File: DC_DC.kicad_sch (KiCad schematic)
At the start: 22 parts, among them Q1 Q_NMOS_GDS, U1 UC3845_SOIC8

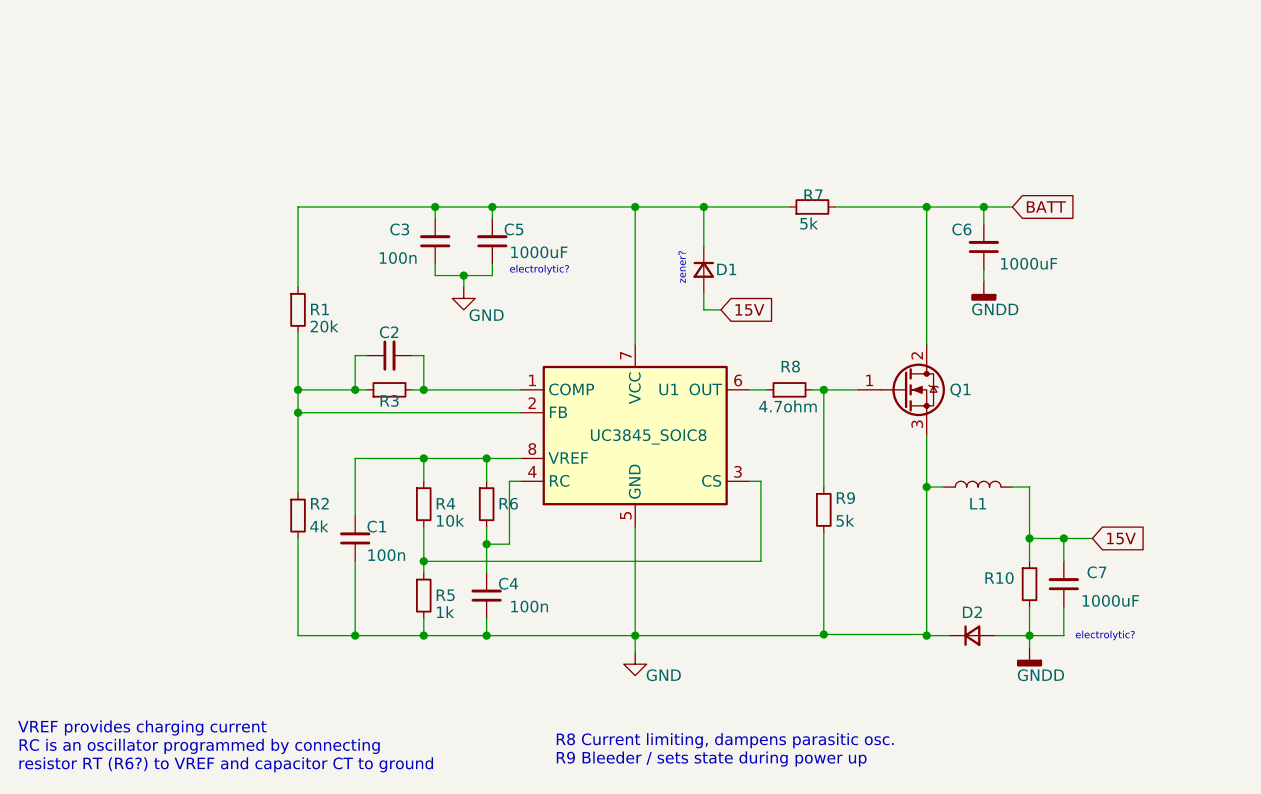
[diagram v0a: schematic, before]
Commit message: thing
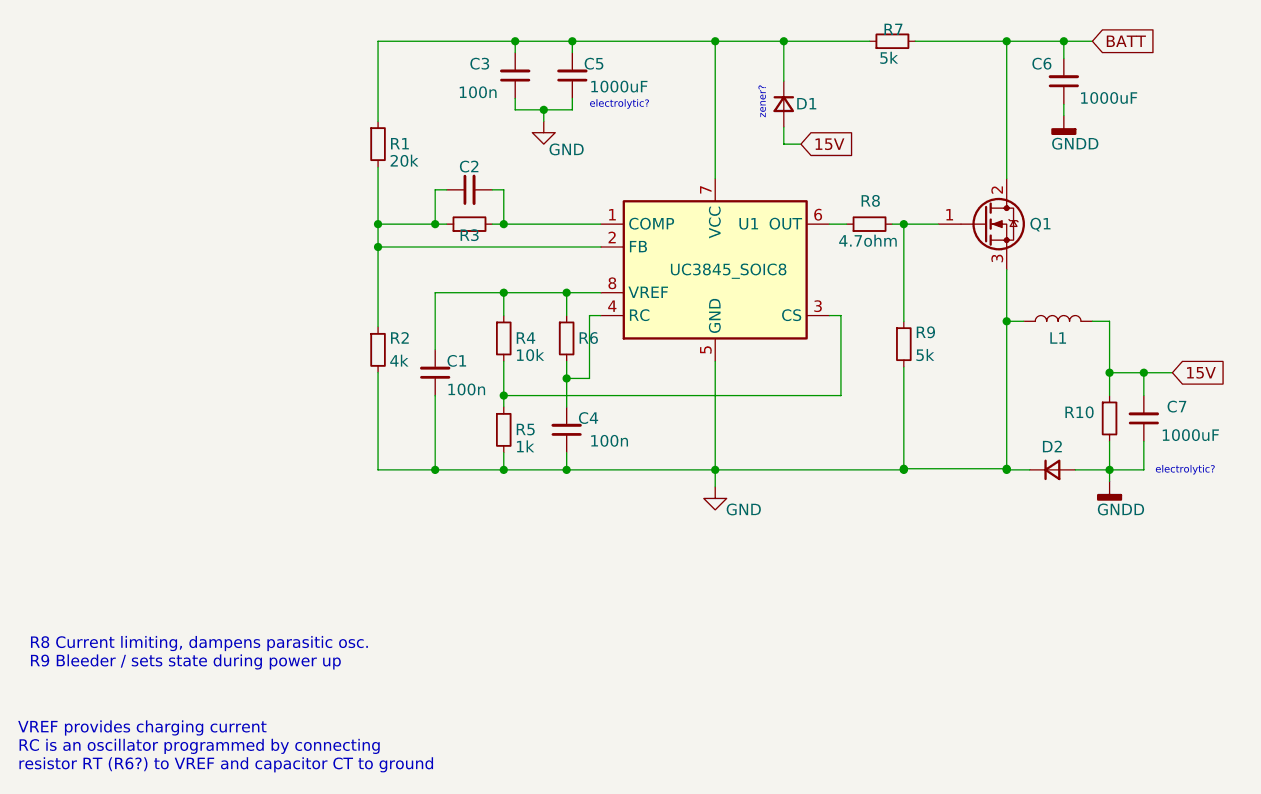
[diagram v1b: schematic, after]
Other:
- moved on the sheet: C1, C2, C3, C4, C5, C6, C7, D1, D2, L1, Q1, R1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
